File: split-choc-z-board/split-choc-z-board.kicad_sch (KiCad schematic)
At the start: 45 parts, among them P2 USB_C_Plug_USB2.0, SW1 SW_SPST, SW10 SW_SPST, SW11 SW_SPST, SW12 SW_SPST, SW13 SW_SPST, SW14 SW_SPST, SW15 SW_SPST, SW16 SW_SPST, SW17 SW_SPST, SW18 SW_SPST, SW2 SW_SPST, SW3 SW_SPST, SW4 SW_SPST, SW5 SW_SPST, SW6 SW_SPST, SW7 SW_SPST, SW8 SW_SPST, SW9 SW_SPST, U1 USBLC6-2SC6

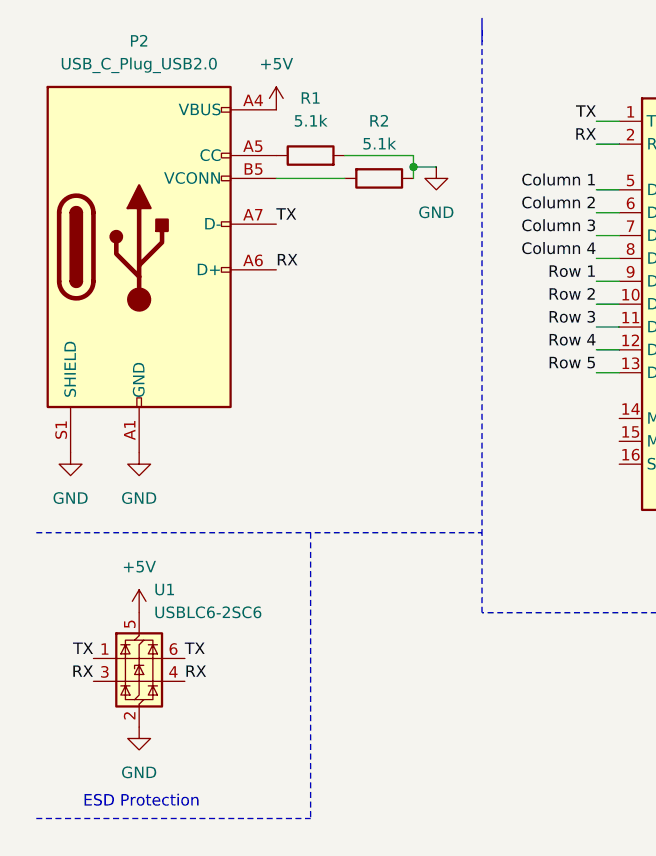
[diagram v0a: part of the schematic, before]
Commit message: Update: Added more footprints 🚀
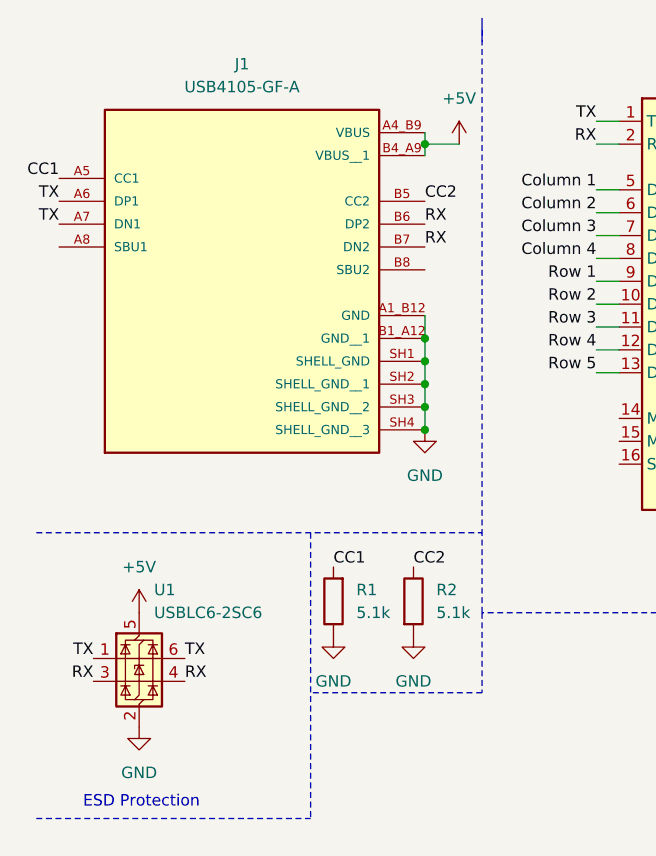
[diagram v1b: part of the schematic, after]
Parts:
- removed P2: USB_C_Plug_USB2.0, symbol Connector:USB_C_Plug_USB2.0
- added J1: USB4105-GF-A, Library:GCT_USB4105-GF-A, symbol USB4105-GF-A:USB4105-GF-A
- D1, D10, D11, D12, D13, D14, D15, D16, D17, D18, D2, D3, D4, D5, D6, D7, D8, D9: footprint Diode_THT:D_DO-35_SOD27_P7.62mm_Horizontal -> footprints:SOD123_MCC
- R1, R2: footprint (none) -> Resistor_THT:R_Axial_DIN0207_L6.3mm_D2.5mm_P10.16mm_Horizontal
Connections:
- net +5V: now also J1.A4_B9 (VBUS), J1.B4_A9 (VBUS__1)
- net GND: now also R1.1, R2.2, J1.A1_B12 (GND), J1.B1_A12 (GND__1), J1.SH1 (SHELL_GND), J1.SH2 (SHELL_GND__1), J1.SH3 (SHELL_GND__2), J1.SH4 (SHELL_GND__3); no longer R1.2, R2.1
- net RX: now also J1.B6 (DP2), J1.B7 (DN2)
- net TX: now also J1.A6 (DP1), J1.A7 (DN1)
- new net CC1: J1.A5 (CC1), R1.2
- new net CC2: J1.B5 (CC2), R2.1
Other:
- moved on the sheet: R1, R2
